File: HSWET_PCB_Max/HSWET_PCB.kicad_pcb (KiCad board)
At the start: 2 copper layers, 105 x 100.2 mm, 21 parts, among them IC3 PS2565L-1-V-F3-A, IC4 PS2565L-1-V-F3-A, IC5 PS2565L-1-V-F3-A, J1 CON-SOCJ-2155, J2 Conn_01x05, J3 CON-SOCJ-2155, U1 INA260AIPWR, U2 YAAJ_DCDC_StepDown_LM2596, U3 YAAJ_DCDC_StepDown_LM2596

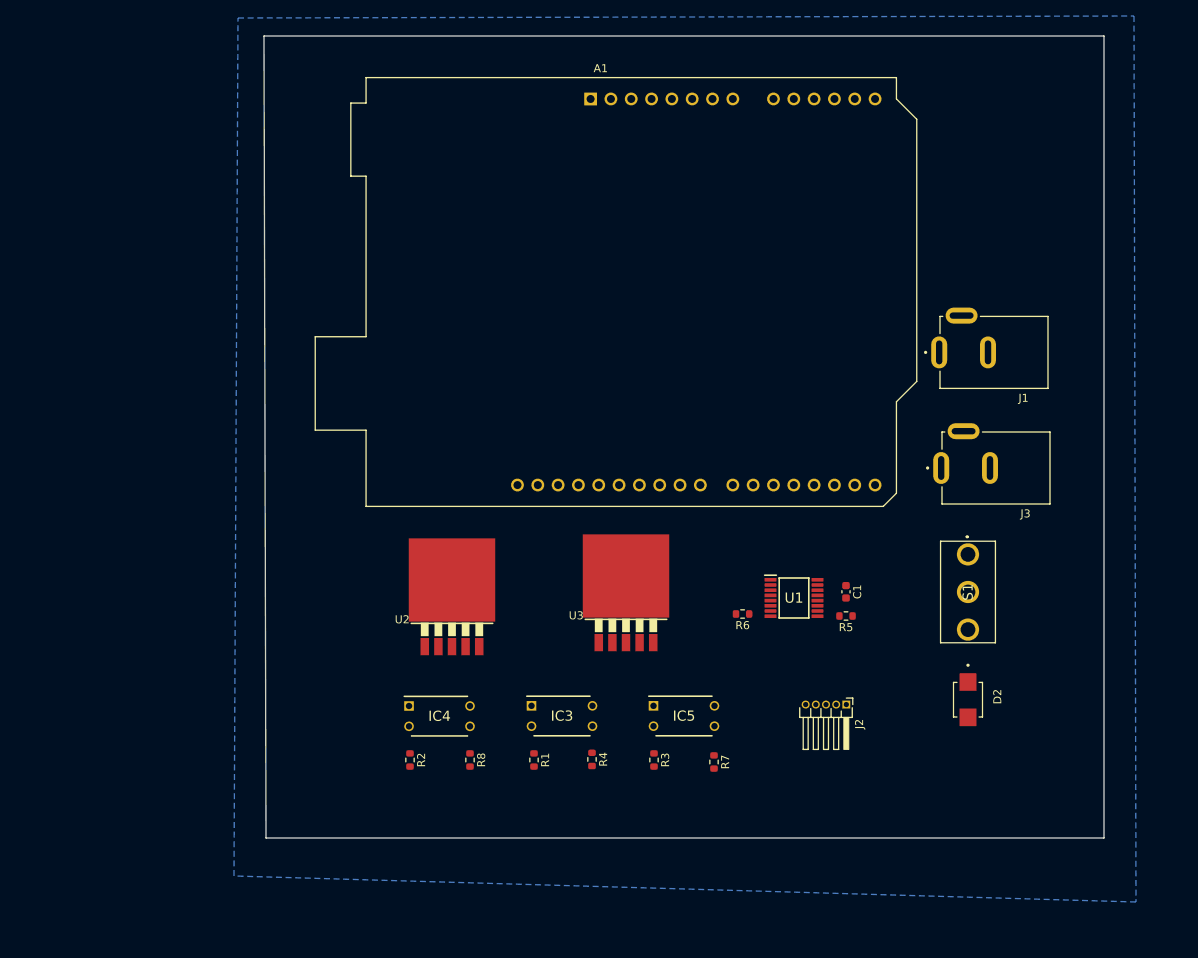
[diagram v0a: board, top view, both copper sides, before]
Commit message: routing done
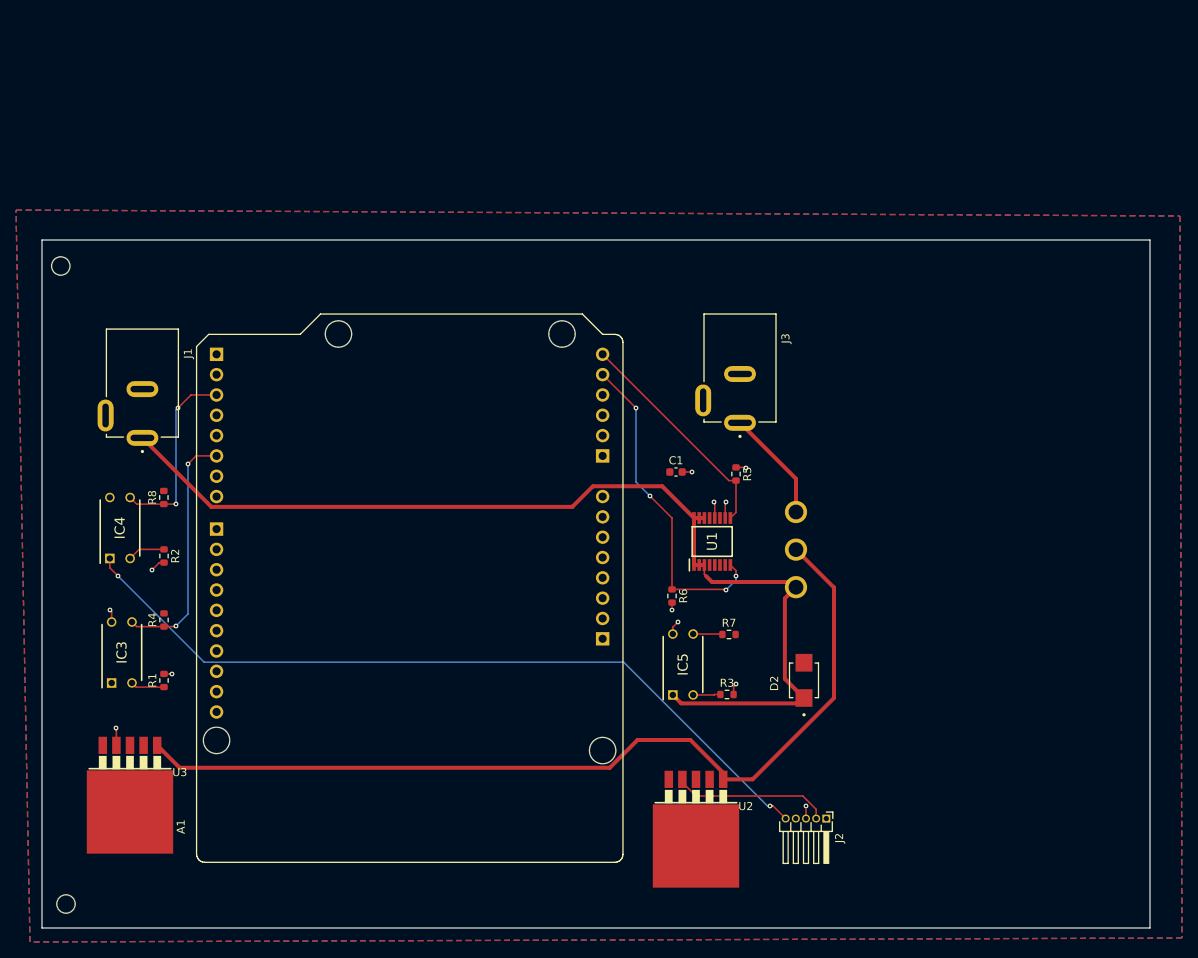
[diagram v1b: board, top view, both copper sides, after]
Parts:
- A1: footprint Module:Arduino_UNO_R3 -> footprints.:ARDUINO_ARDUINO_UNO_REV3
- S1: moved to B.Cu
- moved J1 105.8 mm to (80.3, 67.9), turned to -90 degrees
- moved U3 66.6 mm to (78.8, 118.2), turned to 180 degrees
- moved A1 65.2 mm to (113.7, 92.8), turned to 90 degrees
- moved R4 56.3 mm to (83.0, 96.8), turned to 90 degrees
- moved IC3 55.6 mm to (77.7, 100.8), turned to 90 degrees
- moved R8 50.4 mm to (83.0, 81.4), turned to 90 degrees
- moved R1 47.3 mm to (83.0, 104.3), turned to 90 degrees
- moved IC4 46.4 mm to (77.5, 85.2), turned to 90 degrees
- moved U2 41.5 mm to (149.5, 122.5), turned to 180 degrees
- moved R2 39.9 mm to (83.0, 88.8)
- moved J3 33.4 mm to (155.0, 66.0), turned to -90 degrees
- moved C1 26.0 mm to (147.0, 78.2), turned to 0 degrees
- moved R5 22.5 mm to (154.5, 78.5), turned to -90 degrees
- moved S1 22.1 mm to (162.0, 88.0)
- moved D2 20.6 mm to (163.0, 104.3), turned to 90 degrees
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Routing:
- net Turbine_PWR: track 0.00 -> 129.5 mm
- net Net-(U2-Vin): track 0.00 -> 114.4 mm
- net Turbine_Encoder: track 0.00 -> 98.6 mm, vias 0 -> 2
- net A4: track 0.00 -> 41.1 mm, vias 0 -> 4
- net arduino_lin_act: track 0.00 -> 30.6 mm, vias 0 -> 2
- net A5: track 0.00 -> 28.2 mm
- net arduino_encoder: track 0.00 -> 23.7 mm, vias 0 -> 2
- net 6V: track 0.00 -> 19.6 mm
- net 5V: track 0.00 -> 19.0 mm, vias 0 -> 12
- net 9V: track 0.00 -> 14.0 mm
- net Net-(IC4-CATHODE_ANODE): track 0.00 -> 4.70 mm
- net Net-(IC3-CATHODE_ANODE): track 0.00 -> 4.21 mm
- net Sensor_PWR: track 0.00 -> 3.68 mm
- net Net-(IC5-CATHODE_ANODE): track 0.00 -> 3.43 mm
- added copper zone on B.Cu, net 5V
- added copper zone on F.Cu, net GND
- removed copper zone on B.Cu, net GND
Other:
- board size 105 x 100.2 mm -> 138.5 x 86 mm
